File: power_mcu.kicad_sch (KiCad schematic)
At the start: 28 parts, among them J1 12V_Input, U1 TPS563201, U2 TPS563201

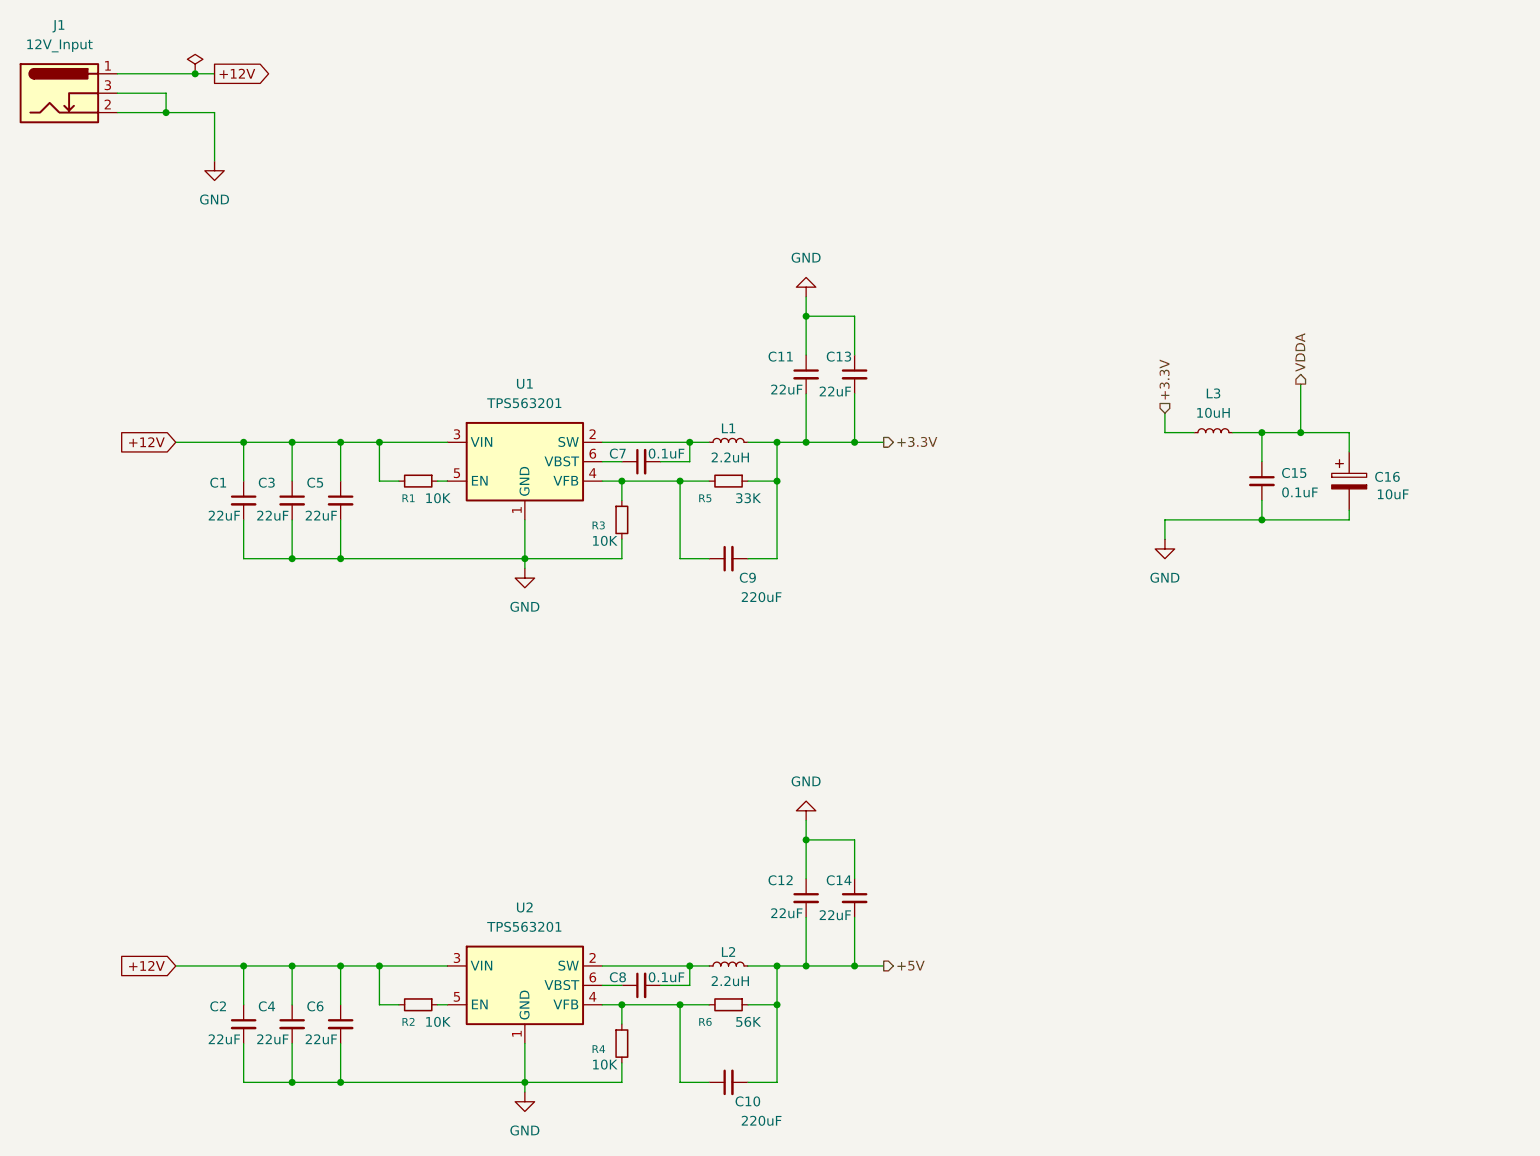
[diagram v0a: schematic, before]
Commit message: update
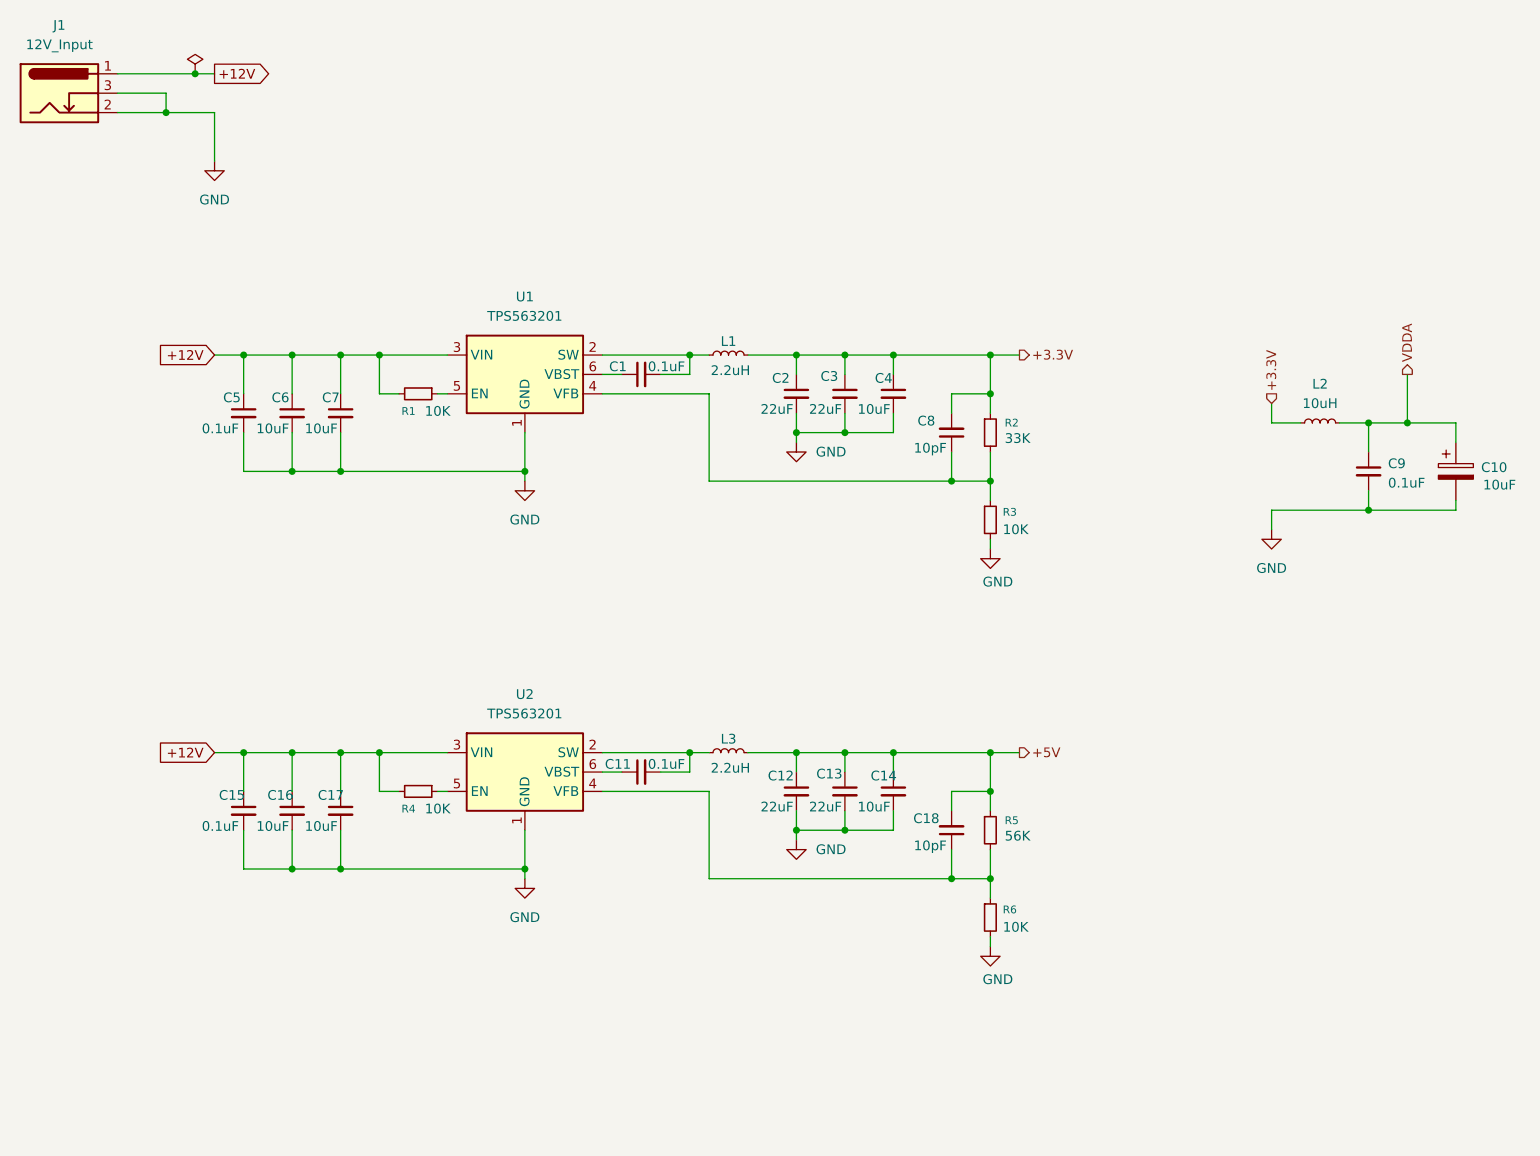
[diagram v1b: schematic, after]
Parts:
- removed C10: 220uF, Capacitor_SMD:C_0603_1608Metric, symbol Device:C_Small
- removed C2, C6: 22uF, Capacitor_SMD:C_0603_1608Metric, symbol Device:C_Small
- removed C8: 0.1uF, Capacitor_SMD:C_0603_1608Metric, symbol Device:C_Small
- removed L2: 2.2uH, Inductor_SMD:L_0603_1608Metric_Pad1.05x0.95mm_HandSolder, symbol Device:L_Small
- removed R2: 10K, Resistor_SMD:R_0603_1608Metric, symbol Device:R_Small
- added C11, C15: 0.1uF, Capacitor_SMD:C_0603_1608Metric, symbol Device:C_Small
- added C13: 22uF, Capacitor_SMD:C_1206_3216Metric, symbol Device:C_Small
- added C16, C17: 10uF, Capacitor_SMD:C_1206_3216Metric, symbol Device:C_Small
- added C18: 10pF, Capacitor_SMD:C_0603_1608Metric, symbol Device:C_Small
- added L3: 2.2uH, Inductor_SMD:L_6.3x6.3_H3, symbol Device:L_Small
- added R5: 56K, Resistor_SMD:R_0603_1608Metric, symbol Device:R_Small
- C12: footprint Capacitor_SMD:C_0603_1608Metric -> Capacitor_SMD:C_1206_3216Metric
- C14, C4: value 22uF -> 10uF; footprint Capacitor_SMD:C_0603_1608Metric -> Capacitor_SMD:C_1206_3216Metric
- C2: renamed from C11; footprint Capacitor_SMD:C_0603_1608Metric -> Capacitor_SMD:C_1206_3216Metric
- C3: renamed from C13; footprint Capacitor_SMD:C_0603_1608Metric -> Capacitor_SMD:C_1206_3216Metric
- C5: renamed from C1; value 22uF -> 0.1uF
- C6: renamed from C3; value 22uF -> 10uF; footprint Capacitor_SMD:C_0603_1608Metric -> Capacitor_SMD:C_1206_3216Metric
- C7: renamed from C5; value 22uF -> 10uF; footprint Capacitor_SMD:C_0603_1608Metric -> Capacitor_SMD:C_1206_3216Metric
- C8: renamed from C9; value 220uF -> 10pF
- L1: footprint Inductor_SMD:L_0603_1608Metric_Pad1.05x0.95mm_HandSolder -> Inductor_SMD:L_6.3x6.3_H3
- R6: value 56K -> 10K
- renumbered C7 to C1, C16 to C10, C15 to C9, L3 to L2, R5 to R2
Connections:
- net +12V: now also R4.2, C15.1, C16.1, C17.1; no longer C4.1
- net +3.3V: now also C2.1, C3.1, C4.1; no longer C2.2, C3.2
- net +5V: now also C12.1, C14.1, C13.1, C18.2, L3.2, R5.1; no longer C12.2, C14.2, R6.1
- net GND: now also C12.2, C14.2, C2.2, C3.2, R6.2, C13.2, C15.2, C16.2, C17.2; no longer C12.1, C14.1, C2.1, C3.1, R4.2
- net at U2.6 (VBST): now also C11.1
- net at U2.2 (SW): now also C11.2, L3.1
- net at U2.5 (EN): now also R4.1
- new net: C18.1, R5.2, R6.1, U2.4 (VFB)
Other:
- moved on the sheet: C1, C10, C2, C3, C5, C6, C7, C8, C9, L1, L2, R1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

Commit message: update
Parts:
- L1, L3: footprint Inductor_SMD:L_6.3x6.3_H3 -> Inductor_SMD:L_Changjiang_FXL0630
- L2: footprint Inductor_SMD:L_0603_1608Metric_Pad1.05x0.95mm_HandSolder -> Inductor_SMD:L_0603_1608Metric
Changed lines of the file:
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@@
 			)
 		)
-		(property "Footprint" "Inductor_SMD:L_6.3x6.3_H3"
+		(property "Footprint" "Inductor_SMD:L_Changjiang_FXL0630"
 			(at 130.81 115.57 0)
 			(effects
@@
 			)
 		)
-		(property "Footprint" "Inductor_SMD:L_0603_1608Metric_Pad1.05x0.95mm_HandSolder"
+		(property "Footprint" "Inductor_SMD:L_0603_1608Metric"
 			(at 208.28 72.39 0)
 			(effects
@@
 			)
 		)
-		(property "Footprint" "Inductor_SMD:L_6.3x6.3_H3"
+		(property "Footprint" "Inductor_SMD:L_Changjiang_FXL0630"
 			(at 130.81 63.5 0)
 			(effects
